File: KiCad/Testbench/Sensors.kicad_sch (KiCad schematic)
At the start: 35 parts, among them J19 Conn_02x02_Top_Bottom, J20 Conn_02x02_Top_Bottom, J21 Conn_02x02_Top_Bottom, J22 Conn_02x02_Top_Bottom, J23 Conn_02x02_Top_Bottom, J24 Conn_02x02_Top_Bottom, J25 Conn_02x02_Top_Bottom, J26 Conn_02x02_Top_Bottom, J27 Conn_02x02_Top_Bottom, J28 Conn_02x02_Top_Bottom

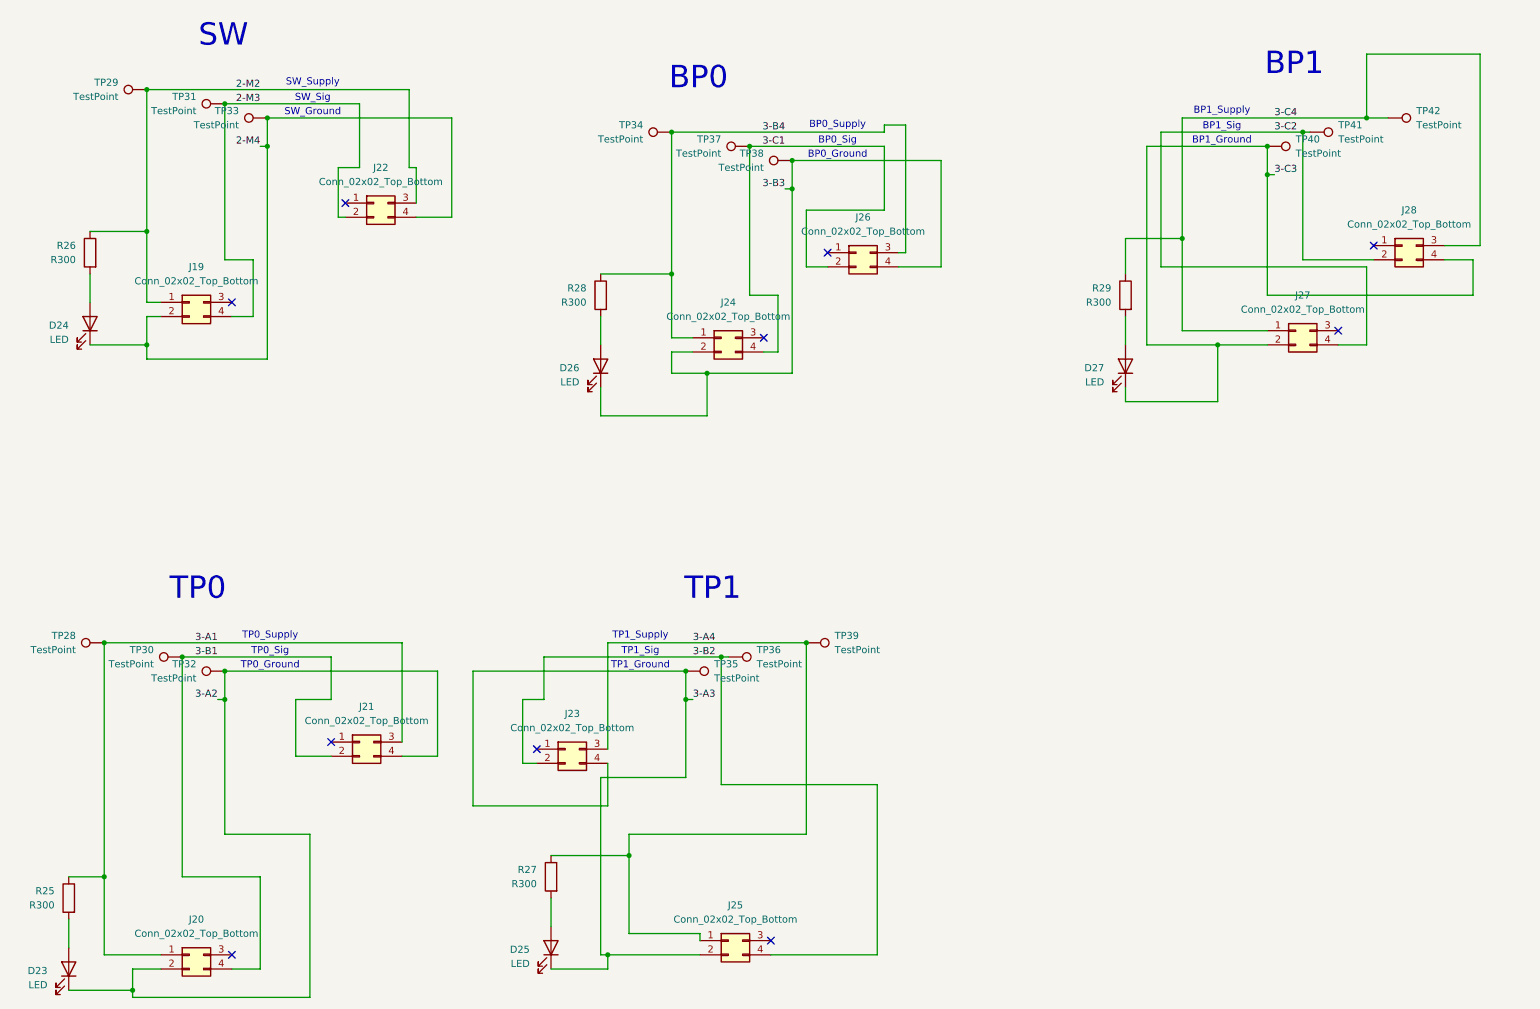
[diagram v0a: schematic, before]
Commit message: After work 151024
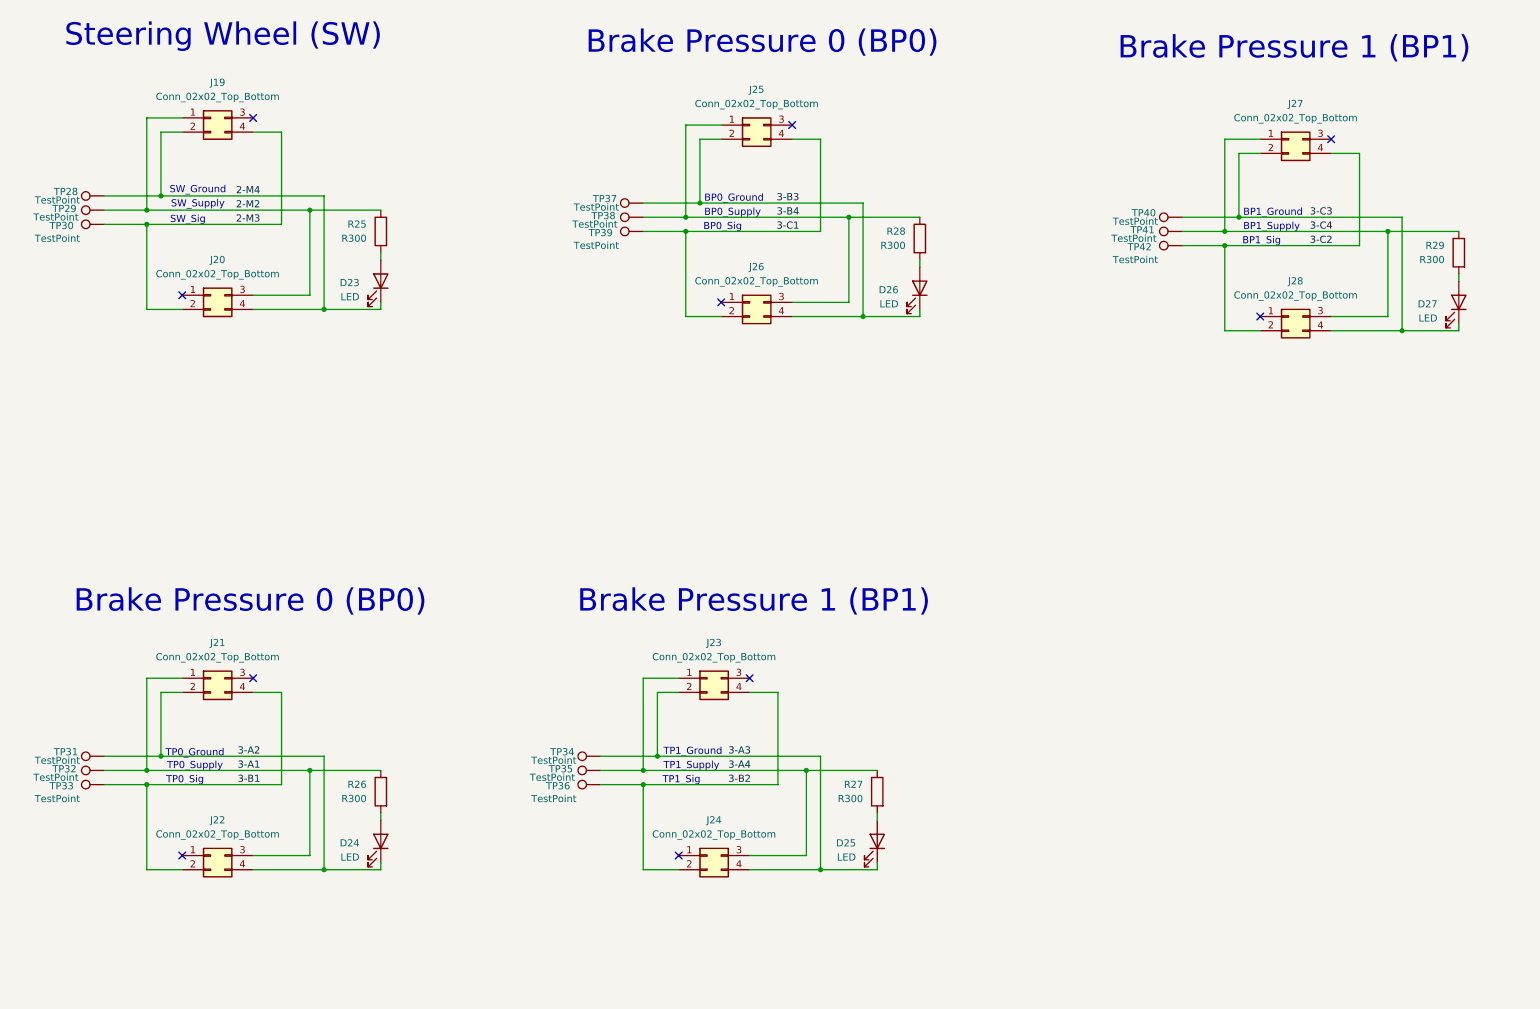
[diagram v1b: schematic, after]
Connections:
- net 2-M2: now also J20.3 (Pin_3), R25.1; no longer J22.3 (Pin_3), R26.1
- net 2-M3: now also J20.2 (Pin_2), TP30.1; no longer J22.2 (Pin_2), TP31.1
- net 2-M4: now also D23.1 (K), J20.4 (Pin_4), TP28.1; no longer D24.1 (K), J22.4 (Pin_4), TP33.1
- net 3-A1: now also J21.1 (Pin_1), J22.3 (Pin_3), R26.1, TP32.1; no longer J20.1 (Pin_1), J21.3 (Pin_3), R25.1, TP28.1
- net 3-A2: now also D24.1 (K), J21.2 (Pin_2), J22.4 (Pin_4), TP31.1; no longer D23.1 (K), J20.2 (Pin_2), J21.4 (Pin_4), TP32.1
- net 3-A3: now also J23.2 (Pin_2), J24.4 (Pin_4), TP34.1; no longer J23.4 (Pin_4), J25.2 (Pin_2), TP35.1
- net 3-A4: now also J23.1 (Pin_1), J24.3 (Pin_3), TP35.1; no longer J23.3 (Pin_3), J25.1 (Pin_1), TP39.1
- net 3-B1: now also J21.4 (Pin_4), J22.2 (Pin_2), TP33.1; no longer J20.4 (Pin_4), J21.2 (Pin_2), TP30.1
- net 3-B2: now also J23.4 (Pin_4), J24.2 (Pin_2); no longer J23.2 (Pin_2), J25.4 (Pin_4)
- net 3-B3: now also J25.2 (Pin_2), TP37.1; no longer J24.2 (Pin_2), TP38.1
- net 3-B4: now also J25.1 (Pin_1), TP38.1; no longer J24.1 (Pin_1), TP34.1
- net 3-C1: now also J25.4 (Pin_4), TP39.1; no longer J24.4 (Pin_4), TP37.1
- net 3-C2: now also TP42.1; no longer TP41.1
- net 3-C4: now also TP41.1; no longer TP42.1
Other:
- note added: "Brake Pressure 0 (BP0)"
- note added: "Brake Pressure 1 (BP1)"
- note added: "Steering Wheel (SW)"
- note removed: "BP0"
- note removed: "BP1"
- note removed: "SW"
- note removed: "TP0"
- note removed: "TP1"
